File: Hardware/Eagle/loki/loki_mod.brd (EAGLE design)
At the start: 21.9 x 22.9 mm, 36 parts

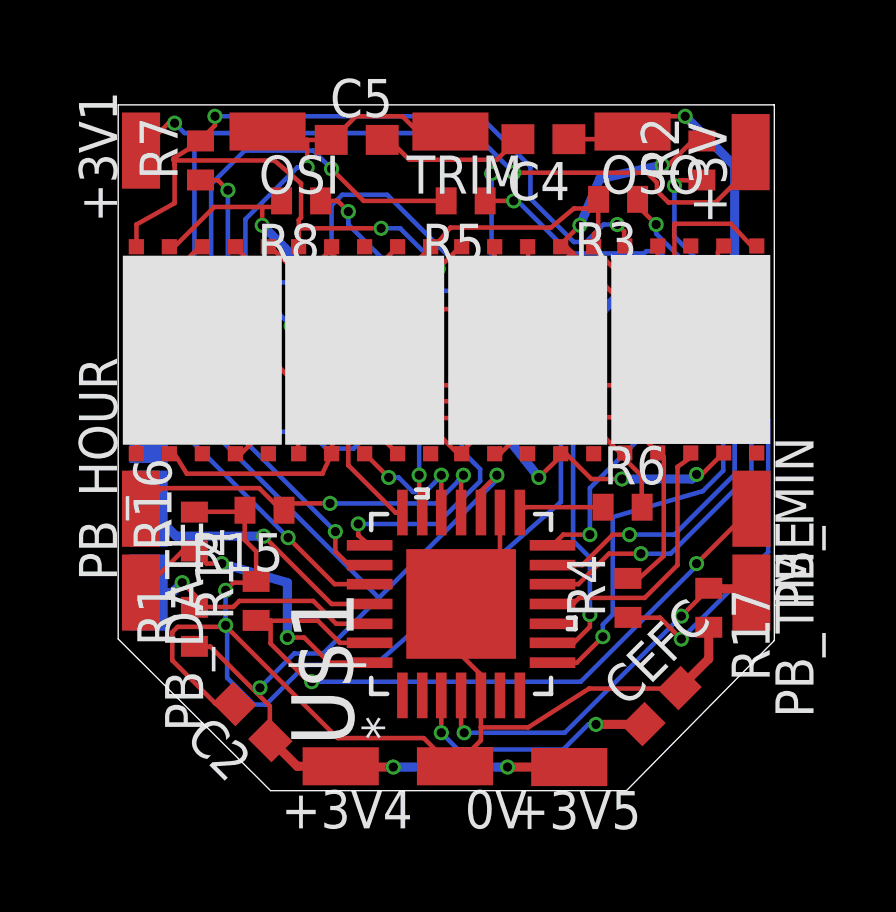
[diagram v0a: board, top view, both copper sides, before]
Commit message: Updated Loki board file.
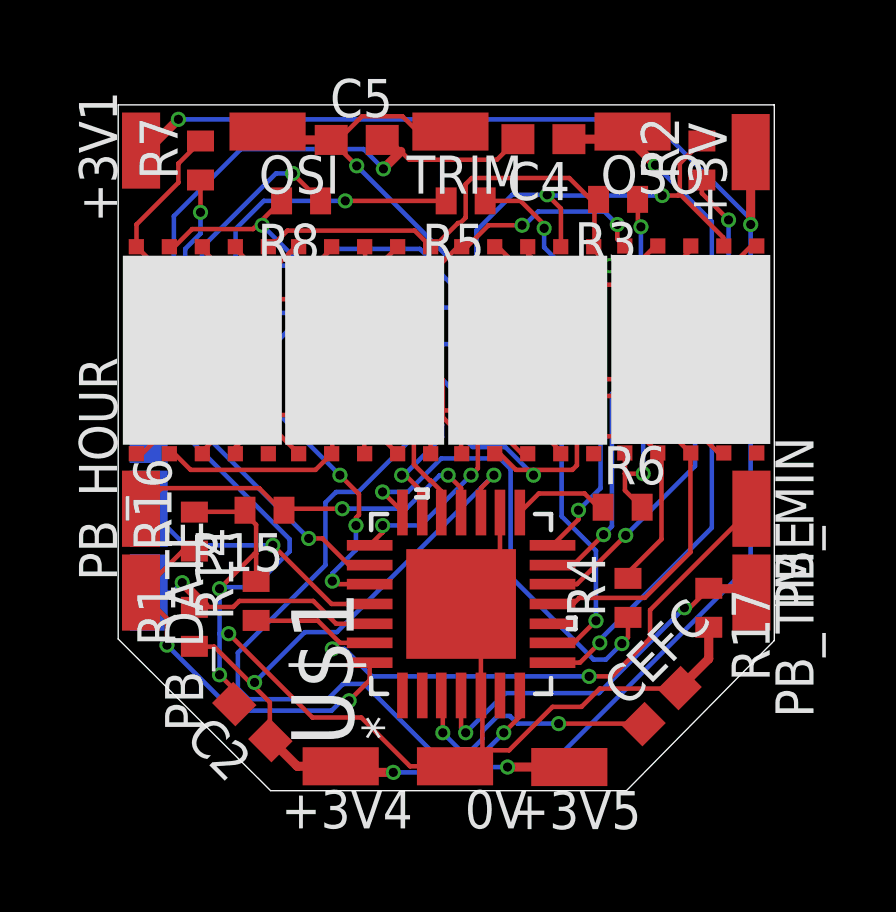
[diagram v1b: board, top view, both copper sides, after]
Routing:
- net OSC2/RA6: track 0.00 -> 24.7 mm, vias 0 -> 2
- net RB3/LED_H3: track 29.5 -> 15.5 mm, vias 4 -> 2
- net N$2: track 35.7 -> 24.4 mm
- net RB1/LED_M6: track 4.57 -> 13.2 mm
- net RB2/LED_H2: track 12.1 -> 20.7 mm, vias 2 -> 4
- net T1OSI: track 36.0 -> 28.2 mm
- net N$9: track 33.6 -> 26.2 mm, vias 5 -> 4
- net RC3/LED_M4: track 8.67 -> 16.0 mm, vias 0 -> 2
- net VDD: track 68.4 -> 74.4 mm
- net PGC/LED_M7: track 16.3 -> 21.5 mm, vias 2 -> 7
- net RC6/LED_M1: track 18.6 -> 14.4 mm
- net RC4/LED_M3: track 20.8 -> 16.7 mm, vias 6 -> 4
- net N$10: track 25.6 -> 21.6 mm
- net GND: track 74.1 -> 70.2 mm, vias 5 -> 4
- net N$13: track 38.4 -> 42.1 mm, vias 9 -> 5
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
